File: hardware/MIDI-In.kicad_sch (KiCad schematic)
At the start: 6 parts, among them J1001 SJ2-25404B-SMT-TR, U1001 TLP2361

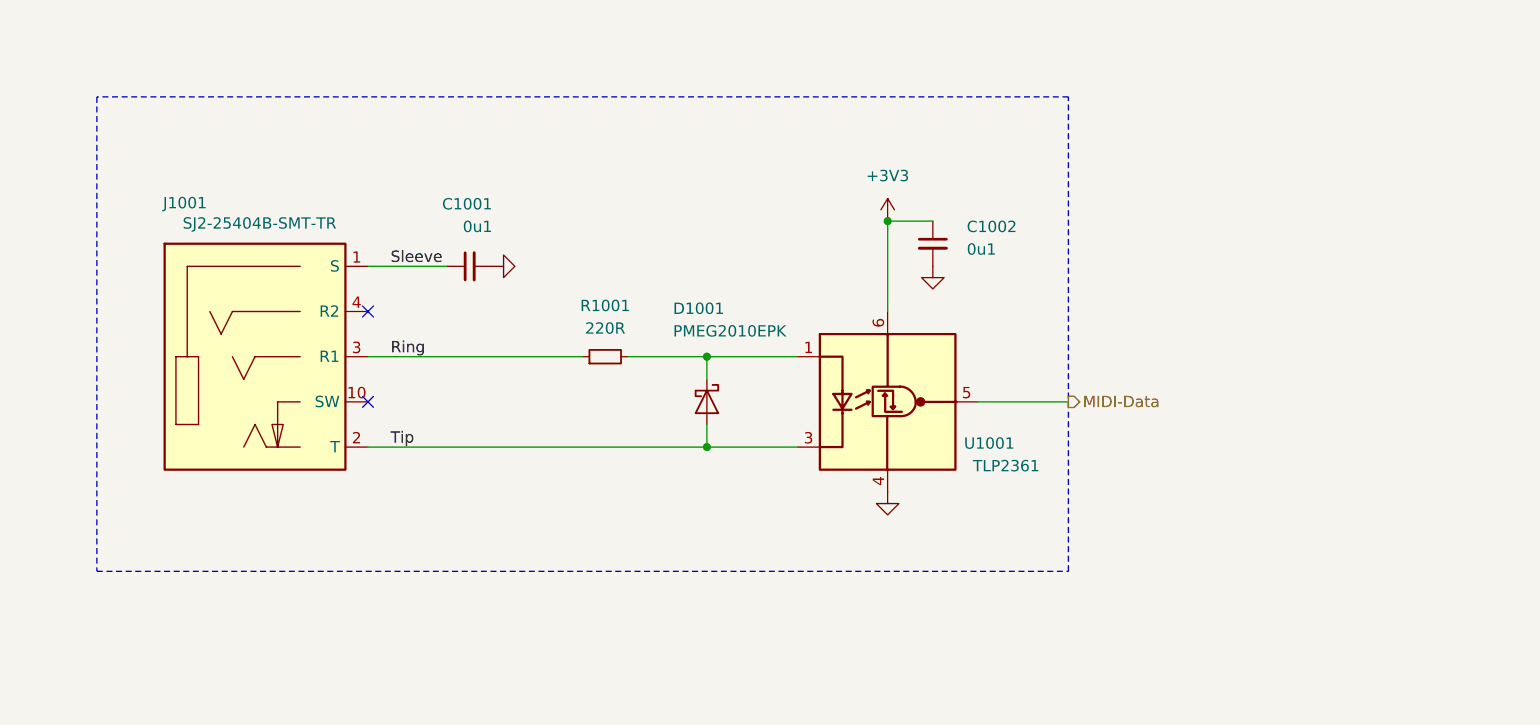
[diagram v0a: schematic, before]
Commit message: Move parts away from edge
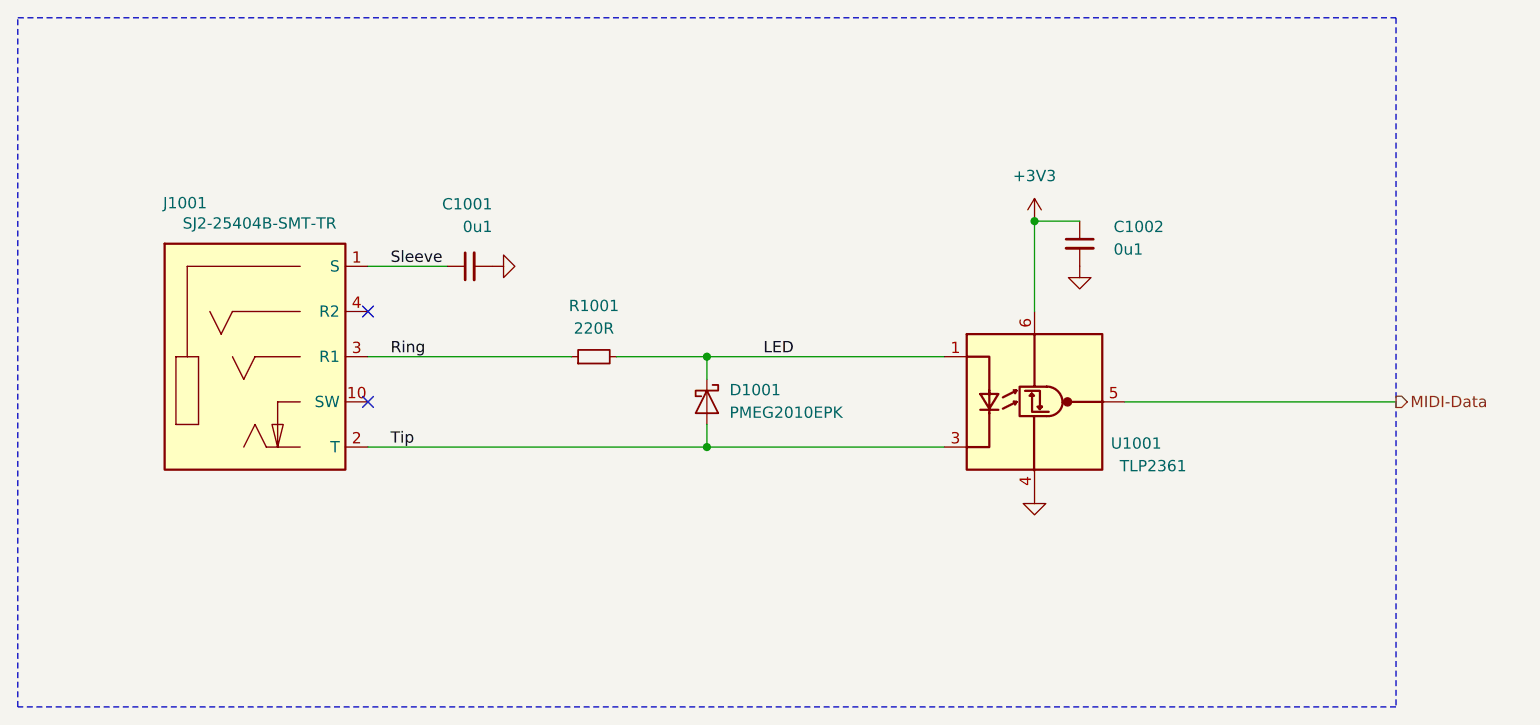
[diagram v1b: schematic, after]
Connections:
- net LED: now reaches D1001.1 (K), R1001.2, U1001.1 (A)
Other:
- moved on the sheet: C1002, R1001, U1001
